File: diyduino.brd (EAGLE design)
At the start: 57.1 x 53.3 mm, 20 parts

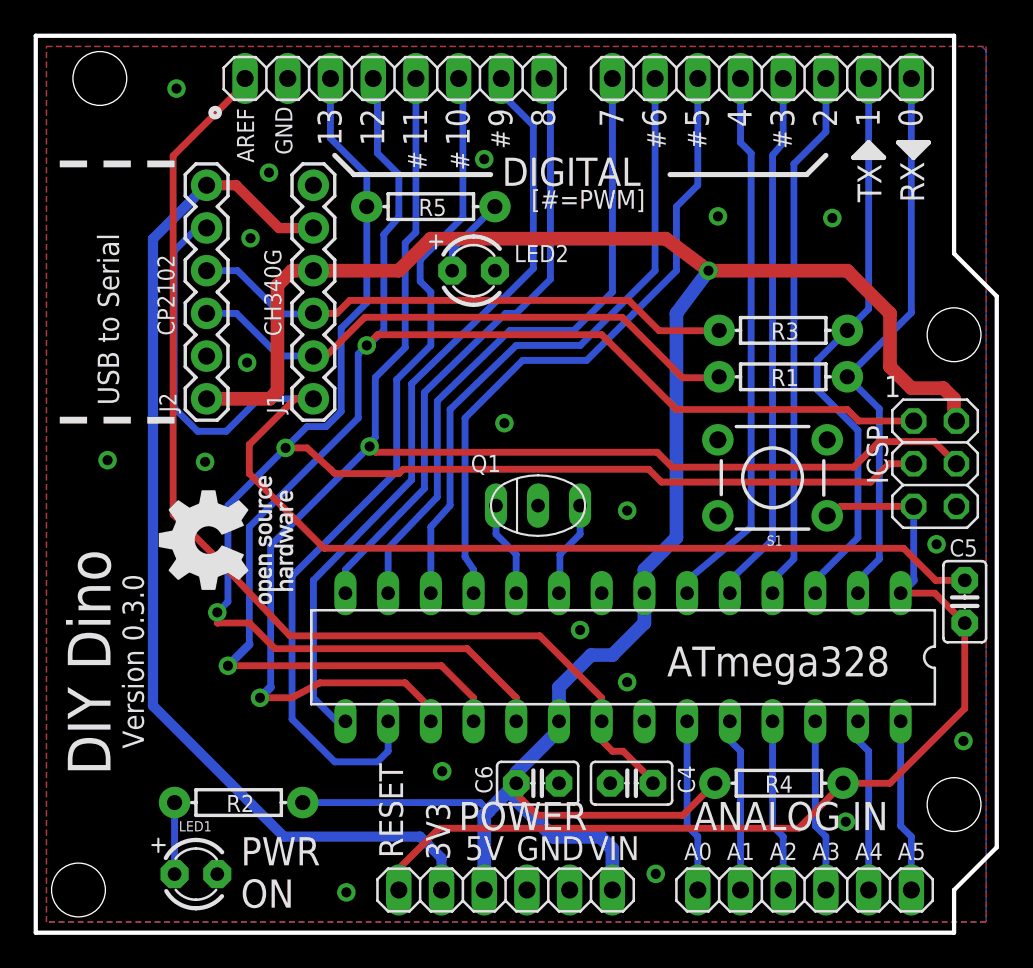
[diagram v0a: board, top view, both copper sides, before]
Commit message: adding dinosaur!
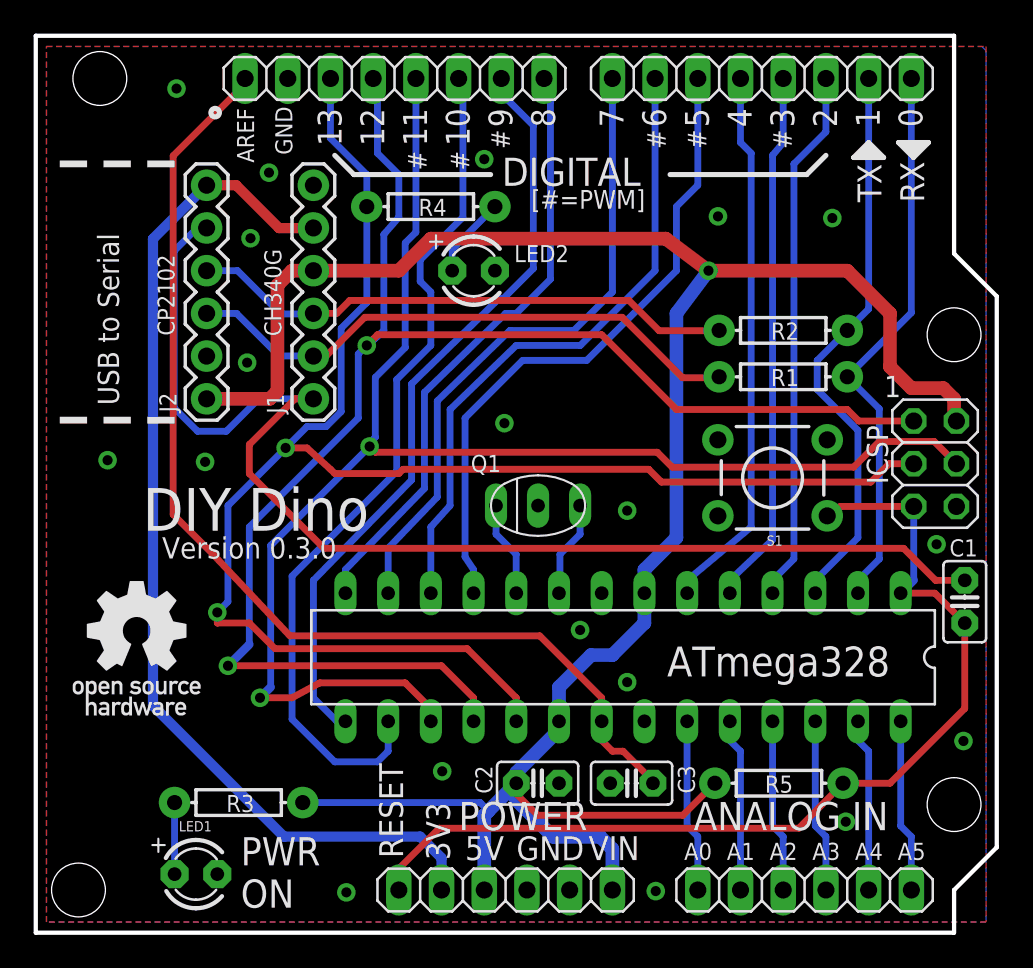
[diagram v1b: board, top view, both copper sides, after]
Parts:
- moved R2 42.9 mm to (55.9, 35.8), turned to 0 degrees
- moved R3 42.9 mm to (23.5, 7.74), turned to 180 degrees
- moved R4 40.1 mm to (34.9, 43.2), turned to 0 degrees
- moved R5 40.1 mm to (55.6, 8.89), turned to 180 degrees
- renumbered C4 to C3, C5 to C1, C6 to C2
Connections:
- net +5V: now also R3.P$1, R5.P$2; no longer R2.P$1, R4.P$2
- net IO1: now also R2.P$2; no longer R3.P$2
- net M8TXD: now also R2.P$1; no longer R3.P$1
- net N$1: now also R4.P$2; no longer R5.P$2
- net N$2: now also R3.P$2; no longer R2.P$2
- net RESET: now also R5.P$1; no longer R4.P$1
- net SCK: now also R4.P$1; no longer R5.P$1
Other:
- board text added: "C1"
- board text added: "C2"
- board text added: "C3"
- board text removed: "C4"
- board text removed: "C5"
- board text removed: "C6"
